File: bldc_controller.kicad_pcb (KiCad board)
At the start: 4 copper layers, 102.9 x 105.4 mm, 151 parts, among them J1 Conn_01x06_Male, Q1 2N7002E, Q10 IRLB8721PBF, Q11 IRLB8721PBF, Q2 DMN65D8L-7, Q3 DMN65D8L-7, Q4 MMBT3904, Q5 IRF4905, Q6 IRLB8721PBF, Q7 IRLB8721PBF, Q8 IRLB8721PBF, Q9 IRLB8721PBF, SW1 1301.9314, SW2 D6C50 F1 LFS, SW3 D6C40 F1 LFS, U1 ATmega328P-PU, U10 IRS2004, U2 SN74LVC1G11DBVR, U3 uA7810, U4 LM7805_TO220, U5 CD4044BE, U6 LM339, U7 MCP601-xP, U8 IRS2004, U9 IRS2004, Y1 9B-16.000MBBK-B

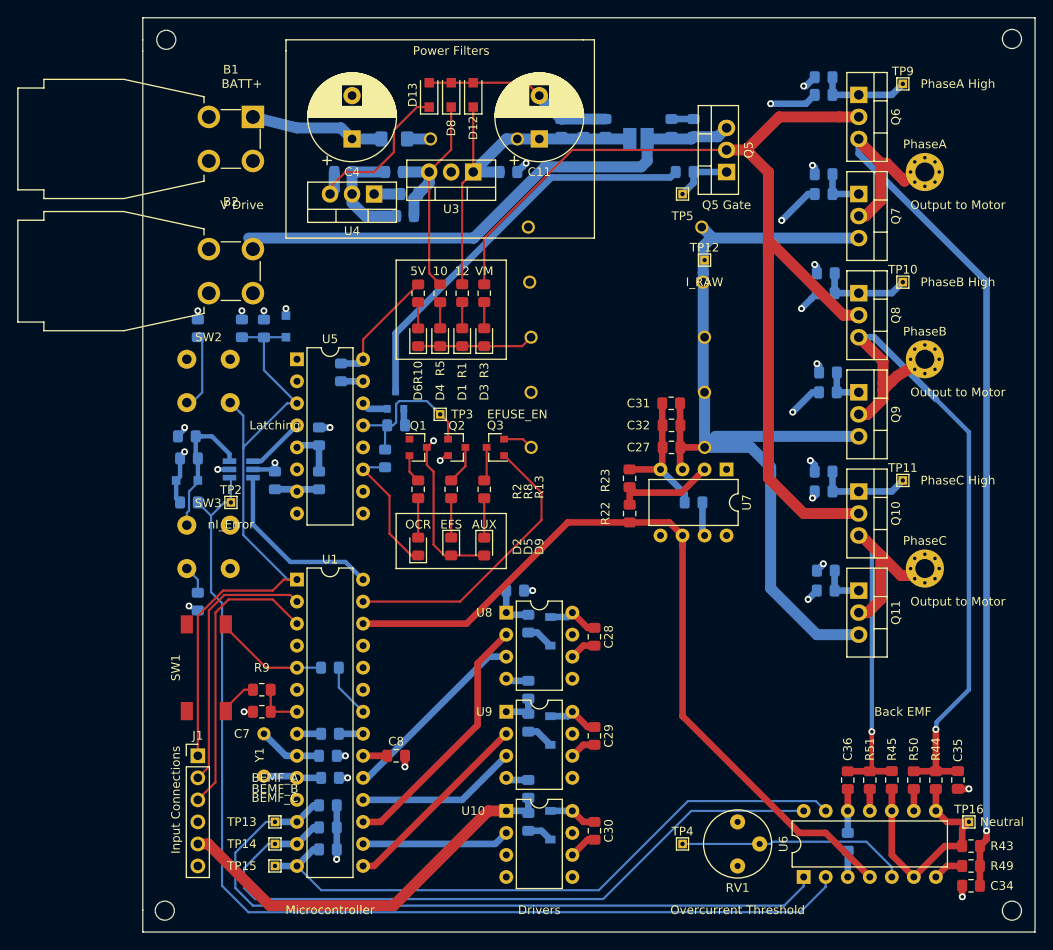
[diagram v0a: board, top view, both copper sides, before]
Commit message: Manual Revert
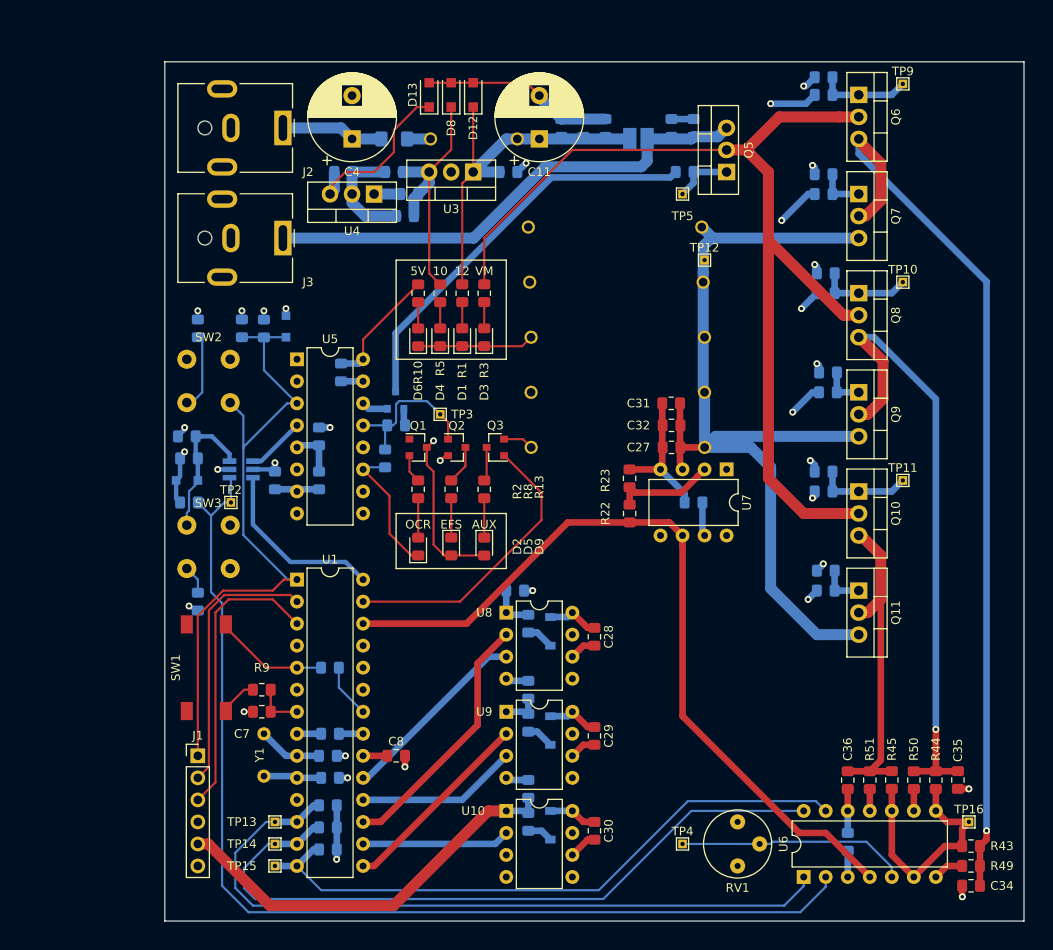
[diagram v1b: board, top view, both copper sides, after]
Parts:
- removed B1: Banana_Jack, Connector:CalTest_CT3151
- removed B2: CalTest_CT3151, Connector:CalTest_CT3151
- removed MH1: MountingHole_Top_Left, MountingHole:MountingHole_2.2mm_M2
- removed MH2: MountingHole_Top_Right, MountingHole:MountingHole_2.2mm_M2
- removed MH3: MountingHole_Bottom_Right, MountingHole:MountingHole_2.2mm_M2
- removed MH4: MountingHole_Bottom_Left, MountingHole:MountingHole_2.2mm_M2
- removed PhaseA, PhaseB, PhaseC: MountingHole_2.2mm_M2_Pad_Via, MountingHole:MountingHole_2.2mm_M2_Pad_Via
- added J2: Banana_Jack, Connector_BarrelJack:BarrelJack_CUI_PJ-063AH_Horizontal, F.Cu at (114.0, 48.3)
- added J3: Banana_Jack, Connector_BarrelJack:BarrelJack_CUI_PJ-063AH_Horizontal, F.Cu at (114.0, 61.0)
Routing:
- net PhaseC: track 106.7 -> 92.9 mm, vias 1 -> 0
- net PhaseB: track 149.8 -> 139.6 mm
- net PhaseA: track 198.4 -> 190.0 mm
- net +BATT: track 16.8 -> 11.9 mm
- net Vdrive: track 61.8 -> 57.9 mm
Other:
- board size 102.9 x 105.4 mm -> 99.1 x 99.1 mm
- board text removed: "BATT+"
- board text removed: "BEMF_A"
- board text removed: "BEMF_B"
- board text removed: "BEMF_C"
- board text removed: "Back EMF"
- board text removed: "Drivers"
- board text removed: "EFUSE_EN"
- board text removed: "I_RAW"
- board text removed: "Input Connections"
- board text removed: "Latching"
- board text removed: "Microcontroller"
- board text removed: "Neutral"
- board text removed: "Output to Motor"
- board text removed: "Overcurrent Threshold"
- board text removed: "PhaseA High"
- board text removed: "PhaseB High"
- board text removed: "PhaseC High"
- board text removed: "Power Filters"
- board text removed: "Q5 Gate"
- board text removed: "V Drive"
- board text removed: "nI_Error"
